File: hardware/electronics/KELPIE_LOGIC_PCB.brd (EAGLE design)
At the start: 101.6 x 57.1 mm, 56 parts, among them J1 PJ-002A, J3 30_PIN_CONNECTOR_MALEFLEX_CON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, J5 SWITCHCRAFT_PHONEJACK, J6 SWD_CONNECTOR, T2 MCP1825S, U4 SGTL5000_32QFN, U5 23LC1024

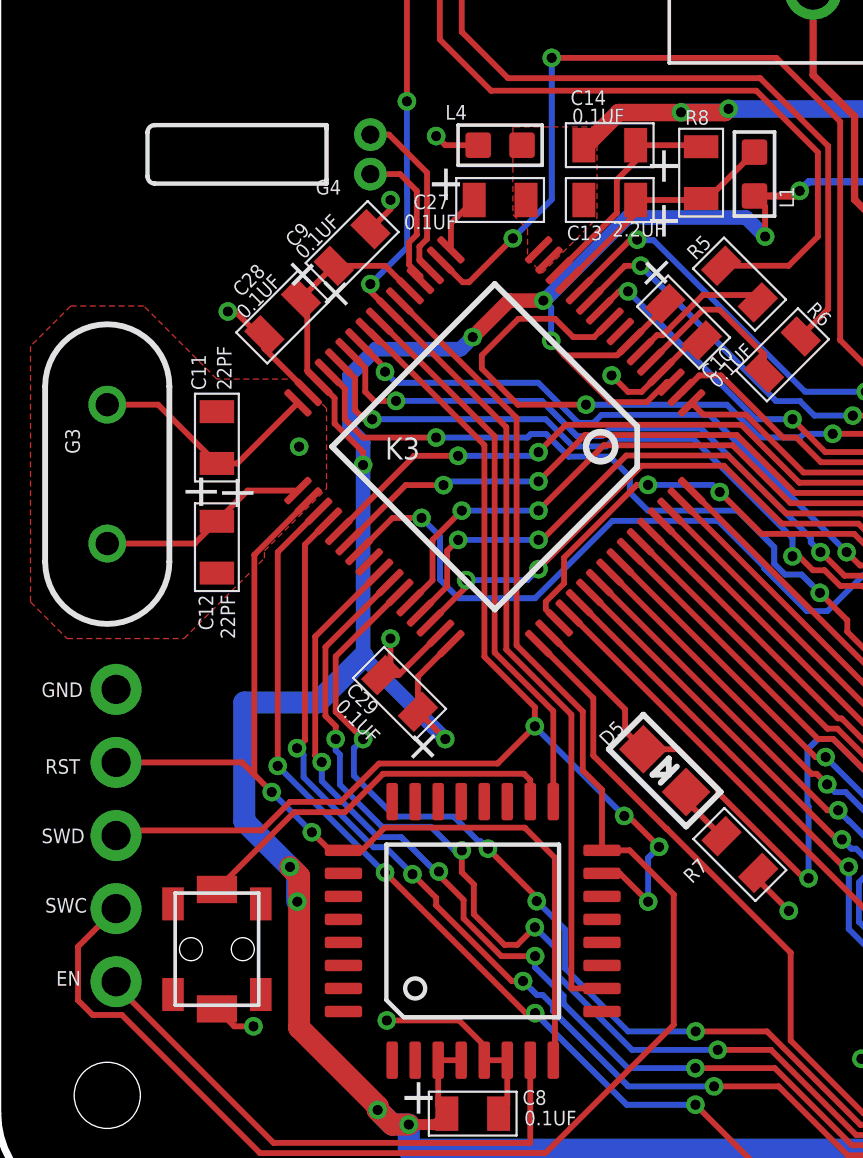
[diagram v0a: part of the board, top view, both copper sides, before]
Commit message: update readme
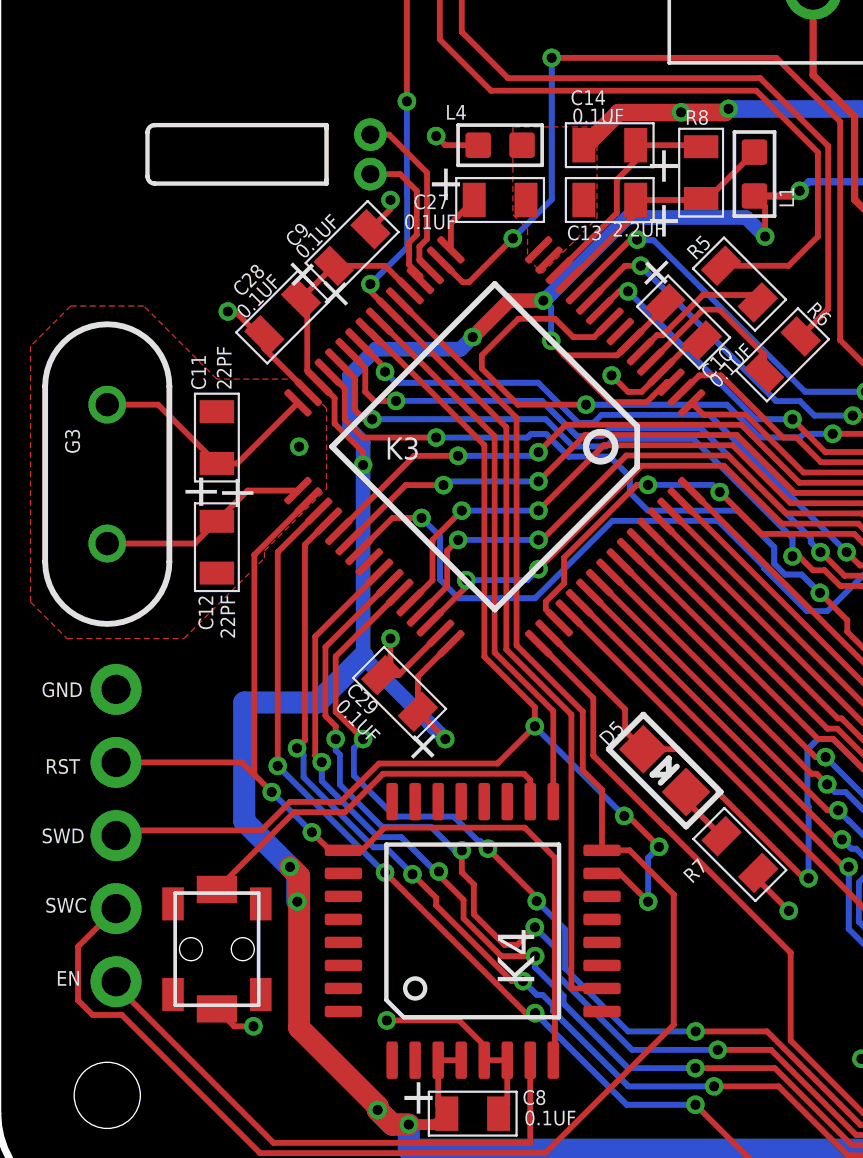
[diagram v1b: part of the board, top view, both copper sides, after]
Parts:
- C11, C12: device moon-germs-v1_main:C_0805 -> sirin-clone-library:C_0805
- D5: device moon-germs-v1_main:CHIPLED_0805 -> sirin-clone-library:CHIPLED_0805
- D6: device moon-germs-v1_main:SOT23-3 -> sirin-clone-library:SOT23-3
- L3, R5, R6, R7, R8: device moon-germs-v1_main:0805 -> sirin-clone-library:0805
- U$6: device moon-germs-v1_main:MICRO-SD-SOCKET -> sirin-clone-library:MICRO-SD-SOCKET
- U4: device moon-germs-v1_main:QFN-32-5MM -> sirin-clone-library:QFN-32-5MM
- U5: device moon-germs-v1_main:TSSOP8 -> sirin-clone-library:TSSOP8

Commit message: hotfix, reexported BOM in BOM folder
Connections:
- net N$20 renamed 1.8V
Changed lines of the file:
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@@
 <drawing>
 <settings>
-<setting alwaysvectorfont="yes"/>
+<setting alwaysvectorfont="no"/>
 <setting verticaltext="up"/>
 </settings>
@@
 </element>
 <element name="C7" library="sirin-clone-library" library_urn="urn:adsk.eagle:library:9336050" package="C_0805" package3d_urn="urn:adsk.eagle:package:8442351/2" value="2.2UF" x="97.79" y="29.21" smashed="yes" rot="R180">
-<attribute name="MPN" value="CL21B105KAFNNNE" x="97.79" y="29.21" size="1.778" layer="27" rot="R180" display="off"/>
+<attribute name="MPN" value="CL21B225KAFNFNE" x="97.79" y="29.21" size="1.778" layer="27" rot="R180" display="off"/>
 <attribute name="NAME" x="96.4692" y="27.7368" size="0.508" layer="21"/>
 <attribute name="VALUE" x="96.4565" y="26.9748" size="0.508" layer="21"/>
@@
 </element>
 <element name="C13" library="sirin-clone-library" library_urn="urn:adsk.eagle:library:9336050" package="C_0805" package3d_urn="urn:adsk.eagle:package:8442351/2" value="2.2UF" x="21.272" y="34.925" smashed="yes" rot="R180">
-<attribute name="MPN" value="CL21B105KAFNNNE" x="21.272" y="34.925" size="1.778" layer="27" rot="R180" display="off"/>
+<attribute name="MPN" value="CL21B225KAFNFNE" x="21.272" y="34.925" size="1.778" layer="27" rot="R180" display="off"/>
 <attribute name="NAME" x="21.018" y="34.036" size="0.508" layer="21" rot="R180"/>
 <attribute name="VALUE" x="23.177" y="34.163" size="0.508" layer="21" rot="R180"/>
@@
 </element>
 <element name="C26" library="sirin-clone-library" library_urn="urn:adsk.eagle:library:9336050" package="C_0805" package3d_urn="urn:adsk.eagle:package:8442351/2" value="2.2UF" x="86.233" y="37.91" smashed="yes">
-<attribute name="MPN" value="CL21B105KAFNNNE" x="86.233" y="37.91" size="1.778" layer="27" display="off"/>
+<attribute name="MPN" value="CL21B225KAFNFNE" x="86.233" y="37.91" size="1.778" layer="27" display="off"/>
 <attribute name="NAME" x="88.011" y="38.1005" size="0.508" layer="21"/>
 <attribute name="VALUE" x="89.8525" y="37.8465" size="0.508" layer="21" rot="R180"/>
@@
 </element>
 <element name="C33" library="sirin-clone-library" library_urn="urn:adsk.eagle:library:9336050" package="C_0805" package3d_urn="urn:adsk.eagle:package:8442351/2" value="2.2UF" x="81.915" y="32.004" smashed="yes" rot="R180">
-<attribute name="MPN" value="CL21B105KAFNNNE" x="81.915" y="32.004" size="1.778" layer="27" rot="R180" display="off"/>
+<attribute name="MPN" value="CL21B225KAFNFNE" x="81.915" y="32.004" size="1.778" layer="27" rot="R180" display="off"/>
 <attribute name="NAME" x="83.566" y="33.401" size="0.508" layer="21" rot="R180"/>
 <attribute name="VALUE" x="80.01" y="32.893" size="0.508" layer="21"/>
 </element>
 <element name="C34" library="sirin-clone-library" library_urn="urn:adsk.eagle:library:9336050" package="C_0805" package3d_urn="urn:adsk.eagle:package:8442351/2" value="2.2UF" x="78.105" y="34.608" smashed="yes" rot="R90">
-<attribute name="MPN" value="CL21B105KAFNNNE" x="78.105" y="34.608" size="1.778" layer="27" rot="R90" display="off"/>
+<attribute name="MPN" value="CL21B225KAFNFNE" x="78.105" y="34.608" size="1.778" layer="27" rot="R90" display="off"/>
 <attribute name="NAME" x="77.6605" y="37.4655" size="0.508" layer="21"/>
 <attribute name="VALUE" x="77.6605" y="36.5765" size="0.508" layer="21"/>
@@
 </element>
 <element name="D6" library="sirin-clone-library" library_urn="urn:adsk.eagle:library:9336050" package="SOT23-3" package3d_urn="urn:adsk.eagle:package:8442353/2" value="AP7313" x="86.36" y="35.242" smashed="yes" rot="R90">
-<attribute name="MPN" value="AP7313-33SRG-7" x="86.36" y="35.242" size="1.778" layer="27" rot="R90" display="off"/>
+<attribute name="MPN" value="AP7313-18SRG-7" x="86.36" y="35.242" size="1.778" layer="27" rot="R90" display="off"/>
 <attribute name="VALUE" x="86.1695" y="36.4485" size="0.508" layer="21" rot="R270"/>
 </element>
@@
 <wire x1="80.3275" y1="41.5925" x2="78.74" y2="43.18" width="0.2032" layer="1"/>
 </signal>
-<signal name="N$20">
+<signal name="1.8V">
 <contactref element="C33" pad="+"/>
 <contactref element="D6" pad="OUT"/>
